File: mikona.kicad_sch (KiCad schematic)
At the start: 0 parts

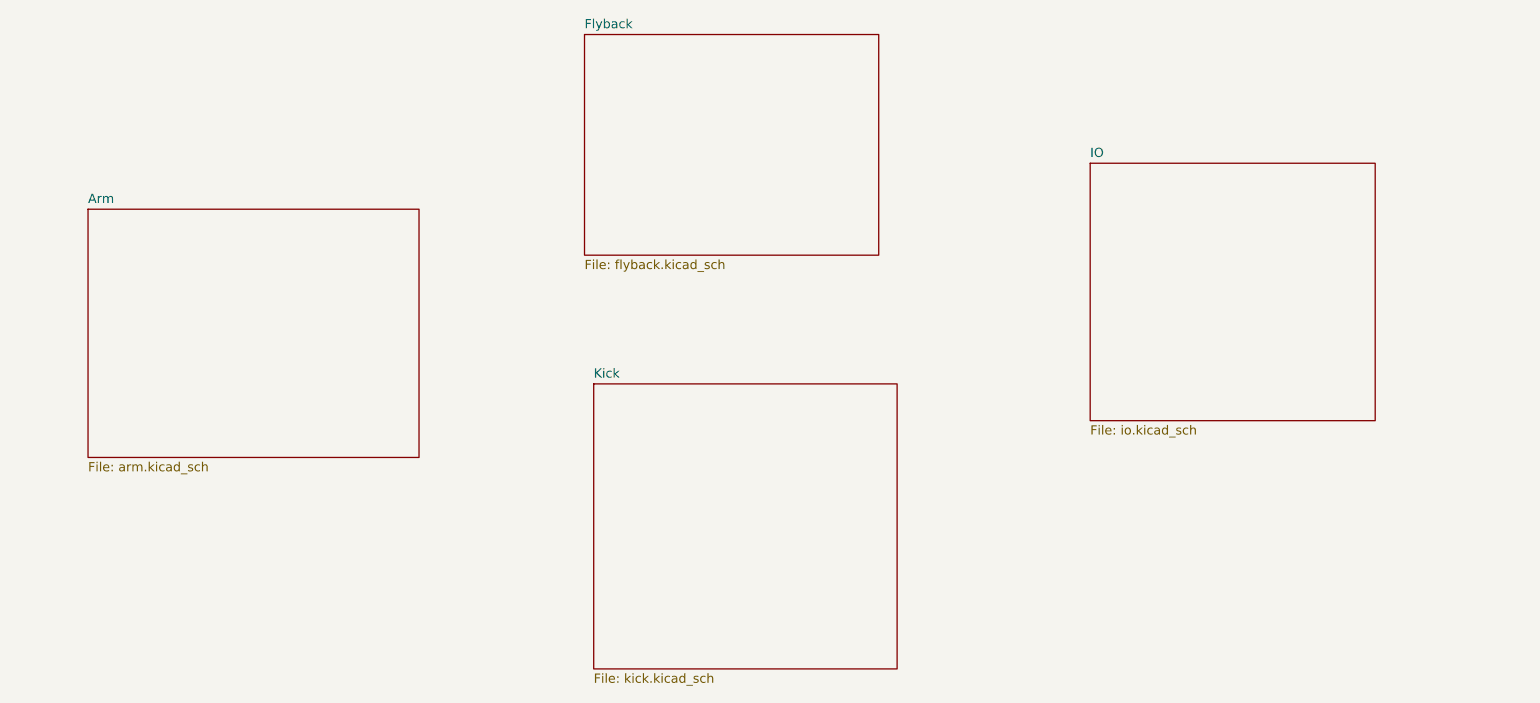
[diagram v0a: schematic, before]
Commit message: Cleanup the project after moving to KiCad.
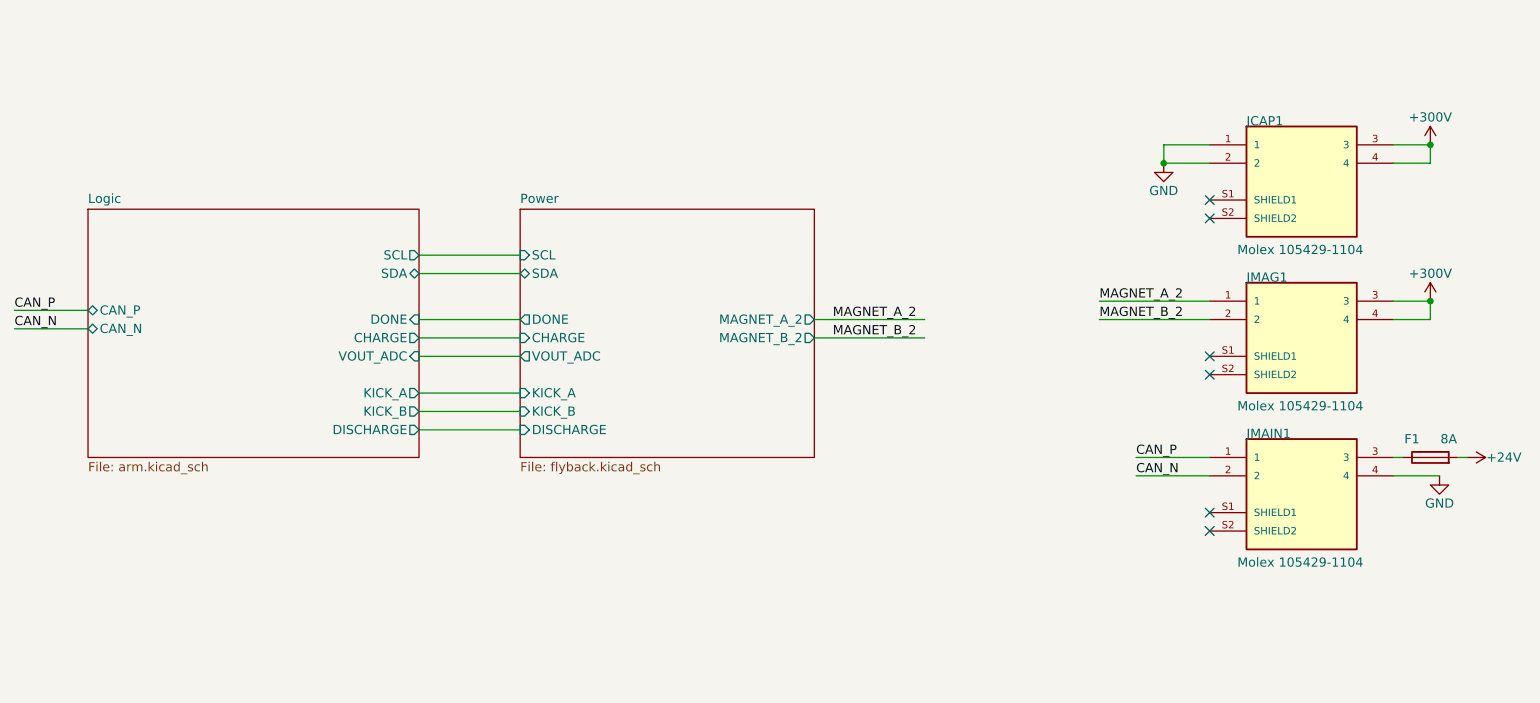
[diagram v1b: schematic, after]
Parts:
- added F1: 8A, Fuse:Fuse_0603_1608Metric_Pad1.05x0.95mm_HandSolder, symbol Device:Fuse
- added JCAP1, JMAG1, JMAIN1: Molex 105429-1104, 1054291104:MOLEX_1054291104, symbol 1054291104:1054291104
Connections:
- new net: F1.1, JMAIN1.3
- new net +24V: F1.2
- new net +3.3V: JCAP1.3, JCAP1.4, JMAG1.3, JMAG1.4
- new net CAN_N: JMAIN1.2
- new net CAN_P: JMAIN1.1
- new net GND: JCAP1.1, JCAP1.2, JMAIN1.4
- new net MAGNET_A_2: JMAG1.1
- new net MAGNET_B_2: JMAG1.2
- no-connect marks 0 -> 6
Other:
- sheet Arm renamed Logic
- sheet Flyback renamed Power
- removed sheet IO
- removed sheet Kick
- sheet Logic ports: added CAN_N, CAN_P, CHARGE, DISCHARGE, DONE, KICK_A, KICK_B, SCL, SDA, VOUT_ADC; removed none
- sheet Power ports: added CHARGE, DISCHARGE, DONE, KICK_A, KICK_B, MAGNET_A_2, MAGNET_B_2, SCL, SDA, VOUT_ADC; removed none
